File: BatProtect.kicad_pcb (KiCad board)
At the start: 2 copper layers, 26.7 x 15.6 mm, 23 parts, among them J1 Bat, J2 Load, Q1 Q_PMOS_GDS, Q2 SI2308, SW1 SW_DIP_x01, U1 ATTINY15-1SC, U2 MIC5219-5.0

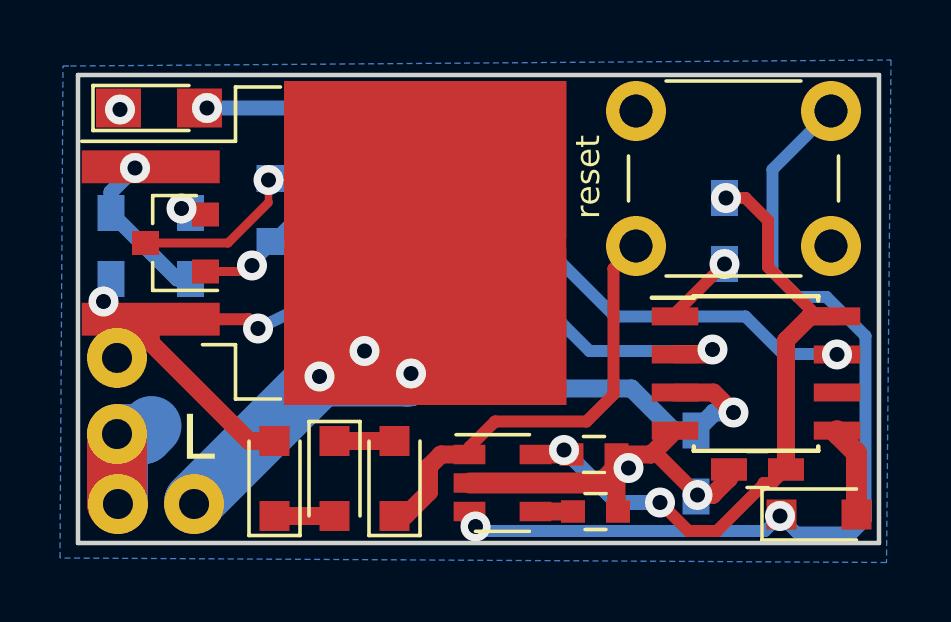
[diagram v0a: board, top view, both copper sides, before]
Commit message: Adjust wierd problem in schematic and add firmware
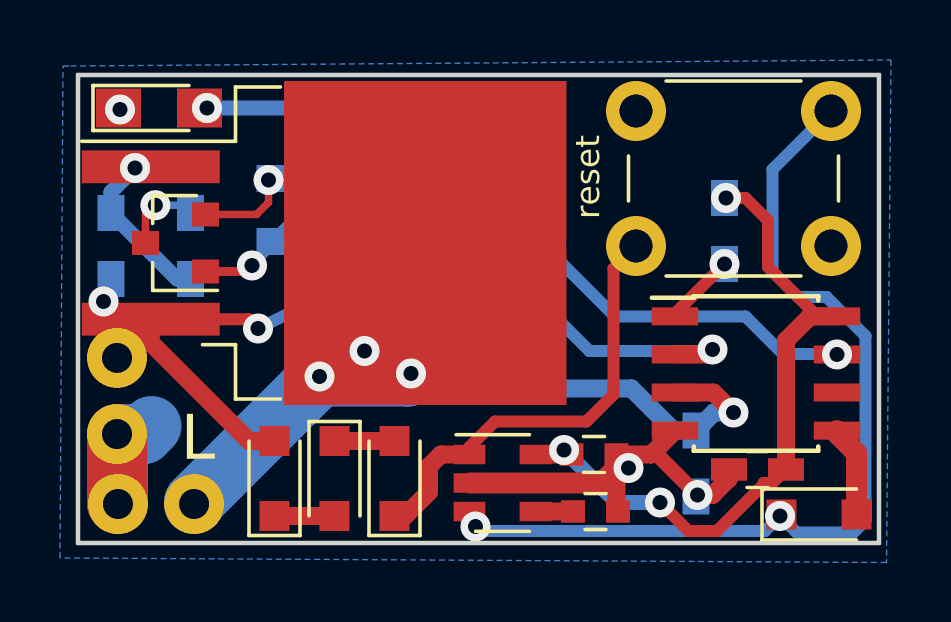
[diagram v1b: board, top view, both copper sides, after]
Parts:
- U1: value ATTINY15-1SC -> ATTINY13A
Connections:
- Q2 pad 2: Net-(Q2-Pad2) -> GND
- Q2 pad 3: GND -> Net-(Q2-Pad3)
- R8 pad 2: Net-(Q2-Pad2) -> Net-(Q2-Pad3)
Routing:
- net Net-(Q2-Pad3): track 0.00 -> 3.14 mm, vias 0 -> 1
- net GND: track 25.3 -> 22.9 mm
- net Net-(Q2-Pad2): track 1.34 -> 0.00 mm, vias 1 -> 0
